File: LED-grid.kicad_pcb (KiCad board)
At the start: 2 copper layers, 75 x 90 mm, 314 parts, among them Q1 NMOS, SW1 SW_Wuerth_450301014042, U1 NE555D, U2 LM741

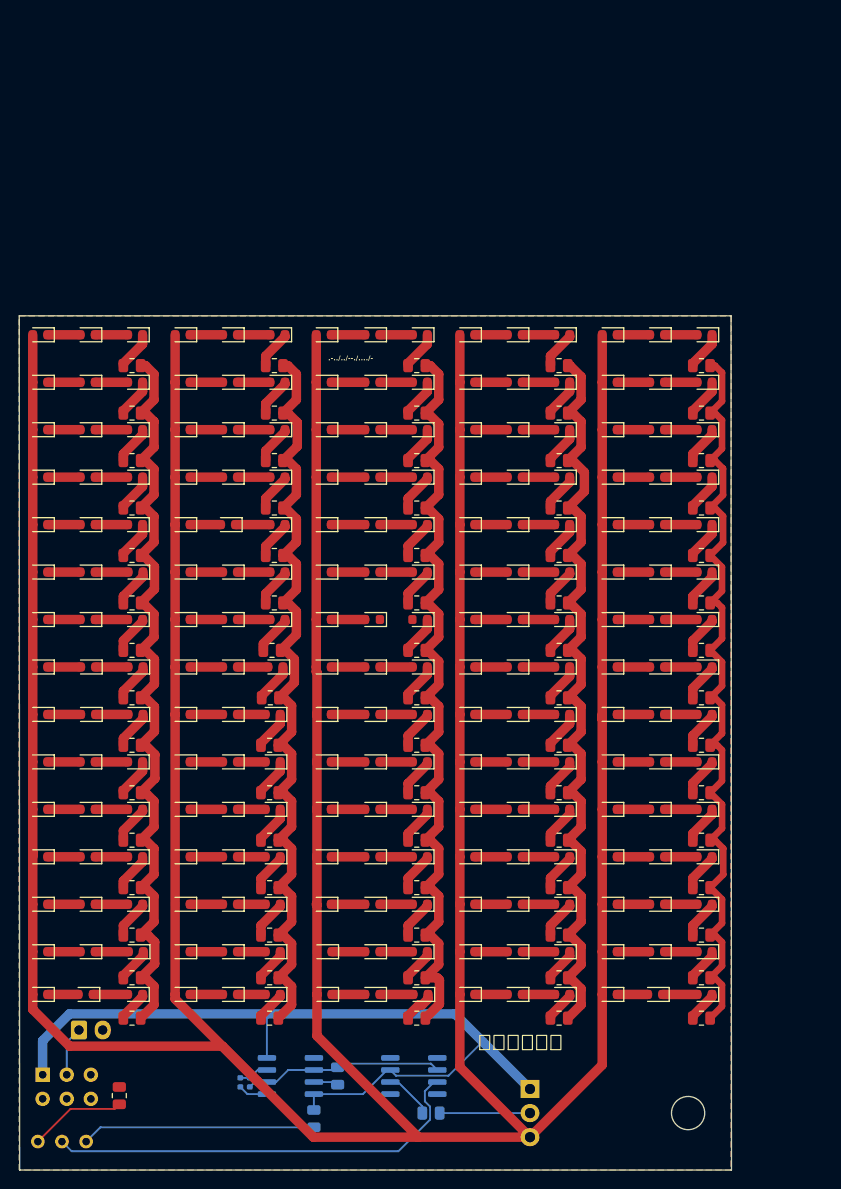
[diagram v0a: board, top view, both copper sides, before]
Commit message: Updated PCB
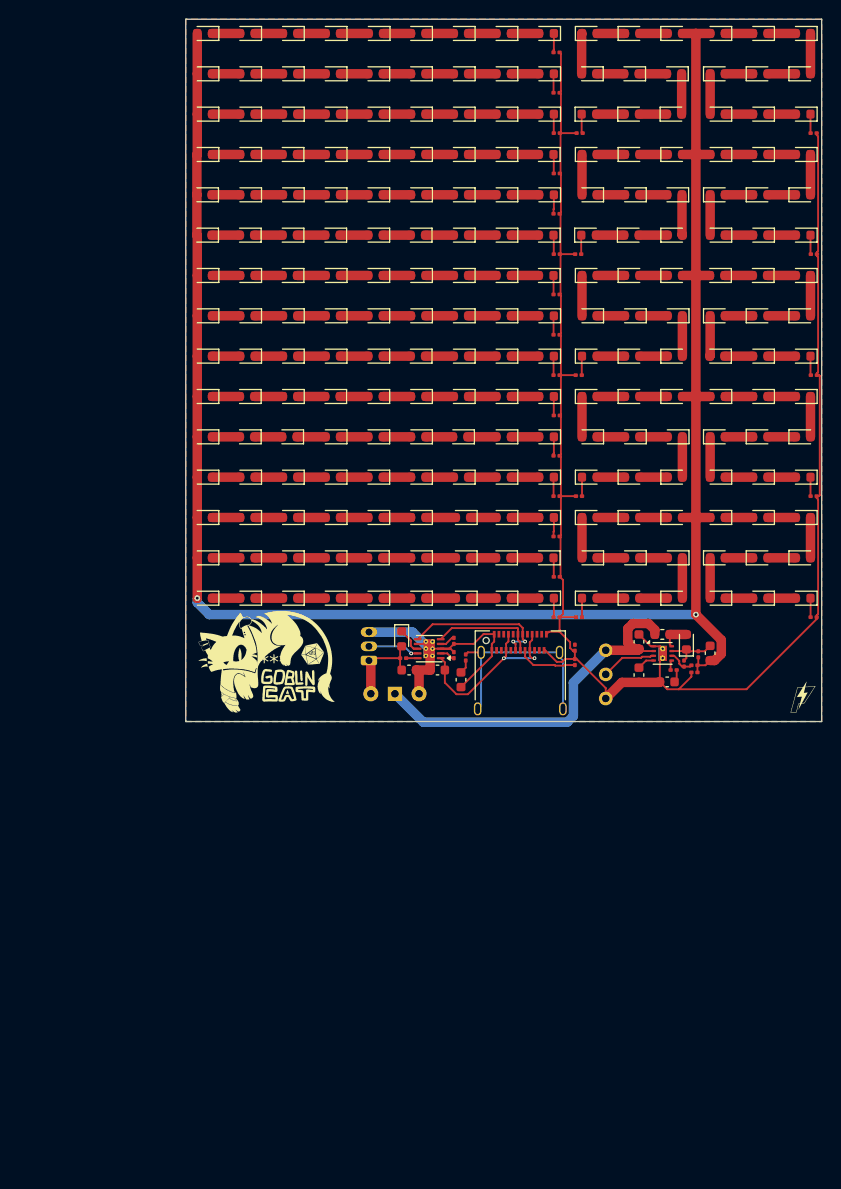
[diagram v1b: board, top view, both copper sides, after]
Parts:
- removed BT1: 6V, Connector_JST:JST_EH_B2B-EH-A_1x02_P2.50mm_Vertical
- removed Q1: NMOS, Package_TO_SOT_THT:TO-220-3_Horizontal_TabUp
- removed R35, R36, R37, R38, R39, R40, R41, R42, R43, R44, R45, R46, R47, R48, R49, R50, R51, R52, R53, R54, R55, R56, R57, R58, R59, R60, R61, R62, R63, R64, R65, R66, R67, R68, R69, R70, R71, R72, R73, R74, R75: 120, Resistor_SMD:R_0805_2012Metric
- removed R76, R77, R78, R79: 1k, Resistor_SMD:R_0805_2012Metric
- removed U2: LM741, Package_SO:SOIC-8_3.9x4.9mm_P1.27mm
- added C3: 1u, Capacitor_SMD:C_0603_1608Metric, F.Cu at (171.0, 92.3)
- added C4: 1u, Capacitor_SMD:C_0603_1608Metric, F.Cu at (195.2, 89.3)
- added C5: 1u, Capacitor_SMD:C_0603_1608Metric, F.Cu at (195.2, 92.8)
- added C6: 10n, Capacitor_SMD:C_0603_1608Metric, F.Cu at (198.2, 93.6)
- added C7: 1n, Capacitor_SMD:C_0201_0603Metric, F.Cu at (200.0, 91.6)
- added C8: 2u, Capacitor_SMD:C_0603_1608Metric, F.Cu at (202.8, 90.5)
- added C9: 47n, Capacitor_SMD:C_0201_0603Metric, F.Cu at (201.1, 92.6)
- added D226: LED, LED_SMD:LED_0603_1608Metric, F.Cu at (208.0, 84.8)
- added D227: LED, LED_SMD:LED_0603_1608Metric, F.Cu at (212.5, 84.8)
- added J1: Conn_01x03_Pin, Connector_JST:JST_ZH_B3B-ZR_1x03_P1.50mm_Vertical, B.Cu at (166.8, 91.3)
- added J2: USB_C_Receptacle, Connector_USB:USB_C_Receptacle_Amphenol_12401610E4-2A, F.Cu at (182.8, 93.6)
- added L1: 30u, Inductor_SMD:L_0603_1608Metric, F.Cu at (197.7, 88.6)
- added U3: BQ24052, Package_SON:WSON-10-1EP_2.5x2.5mm_P0.5mm_EP1.2x2mm_ThermalVias, F.Cu at (173.2, 90.1)
- C1, C2: value 100n -> 1u; footprint Capacitor_SMD:C_0402_1005Metric -> Capacitor_SMD:C_0603_1608Metric; moved to F.Cu
- D2: value LED -> D; footprint LED_SMD:LED_0603_1608Metric -> Diode_SMD:D_0603_1608Metric
- G*** (x2): moved to F.Cu
- R1, R2: value 120 -> 5.1k; footprint Resistor_SMD:R_0805_2012Metric -> Resistor_SMD:R_0201_0603Metric
- R10, R11, R12, R13, R14, R15, R16, R17, R18, R19, R20, R21, R22, R23, R24, R25, R26, R27, R28, R29, R30, R31, R32, R33, R34: value 120 -> 20; footprint Resistor_SMD:R_0805_2012Metric -> Resistor_SMD:R_0201_0603Metric
- R3, R4, R6: value 120 -> 1k; footprint Resistor_SMD:R_0805_2012Metric -> Resistor_SMD:R_0201_0603Metric
- R5: value 120 -> 2k; footprint Resistor_SMD:R_0805_2012Metric -> Resistor_SMD:R_0201_0603Metric
- R7, R8: value 120 -> 100; footprint Resistor_SMD:R_0805_2012Metric -> Resistor_SMD:R_0201_0603Metric
- R9: value 120 -> 1.6; footprint Resistor_SMD:R_0805_2012Metric -> Resistor_SMD:R_0201_0603Metric
- RV1: value 3296X-1-102LF -> 1k
- SW1: footprint Button_Switch_THT:SW_NKK_G1xJP -> Button_Switch_THT:SW_Slide-03_Wuerth-WS-SLTV_10x2.5x6.4_P2.54mm
- U1: value NE555D -> TPS923650D2DRLR; footprint Package_SO:SOIC-8_3.9x4.9mm_P1.27mm -> Package_SON:WSON-8-1EP_2x2mm_P0.5mm_EP0.9x1.6mm_ThermalVias; moved to F.Cu
- moved D183 110.4 mm to (203.5, 25.2)
- moved D184 110.1 mm to (208.0, 25.2)
- moved D196 110.1 mm to (208.0, 42.2), turned to 0 degrees
- moved D185 109.8 mm to (212.5, 25.2)
- moved D186 103.8 mm to (212.5, 29.5), turned to 0 degrees
- moved D197 103.8 mm to (203.5, 42.2), turned to 0 degrees
- moved D187 98.9 mm to (208.0, 29.5), turned to 0 degrees
- moved D211 98.6 mm to (208.0, 63.5)
- moved D212 98.4 mm to (212.5, 63.5)
- moved D198 97.2 mm to (203.5, 46.5)
- moved D199 97.0 mm to (208.0, 46.5)
- moved D200 96.7 mm to (212.5, 46.5)
- moved D138 95.5 mm to (199.0, 25.2), turned to 0 degrees
- moved D188 94.8 mm to (203.5, 29.5), turned to 0 degrees
- moved D213 91.7 mm to (212.5, 67.8), turned to 0 degrees
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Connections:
- C1 pad 1: Net-(U1-CV) -> Net-(C1-Pad1)
- C2 pad 1: Net-(U1-THR) -> VBUS
- D1 pad 2: LED_PWR -> BAT
- D10 pad 2: LED_PWR -> Net-(D10-A)
- D100 pad 2: LED_PWR -> Net-(D100-A)
- D102 pad 2: Net-(D101-K) -> LED_PWR
- D103 pad 2: LED_PWR -> Net-(D102-K)
- D106 pad 2: LED_PWR -> Net-(D105-K)
- D109 pad 2: LED_PWR -> Net-(D108-K)
- D111 pad 2: Net-(D110-K) -> LED_PWR
- D112 pad 2: LED_PWR -> Net-(D111-K)
- D115 pad 2: LED_PWR -> Net-(D114-K)
- D118 pad 2: LED_PWR -> Net-(D117-K)
- D12 pad 2: Net-(D11-K) -> LED_PWR
- D120 pad 2: Net-(D119-K) -> LED_PWR
- D121 pad 2: LED_PWR -> Net-(D120-K)
- D124 pad 2: LED_PWR -> Net-(D123-K)
- D127 pad 2: LED_PWR -> Net-(D126-K)
- D129 pad 2: Net-(D128-K) -> LED_PWR
- D13 pad 2: LED_PWR -> Net-(D12-K)
- D130 pad 2: LED_PWR -> Net-(D129-K)
- D133 pad 2: LED_PWR -> Net-(D132-K)
- D136 pad 2: LED_PWR -> Net-(D135-K)
- D138 pad 2: Net-(D137-K) -> LED_PWR
- D139 pad 2: LED_PWR -> Net-(D138-K)
- D142 pad 2: LED_PWR -> Net-(D141-K)
- D145 pad 2: LED_PWR -> Net-(D144-K)
- D147 pad 2: Net-(D146-K) -> LED_PWR
- D148 pad 2: LED_PWR -> Net-(D147-K)
- D151 pad 2: LED_PWR -> Net-(D150-K)
- D154 pad 2: LED_PWR -> Net-(D153-K)
- D156 pad 2: Net-(D155-K) -> LED_PWR
- D157 pad 2: LED_PWR -> Net-(D156-K)
- D16 pad 2: LED_PWR -> Net-(D15-K)
- D160 pad 2: LED_PWR -> Net-(D159-K)
- D163 pad 2: LED_PWR -> Net-(D162-K)
- D165 pad 2: Net-(D164-K) -> LED_PWR
- D166 pad 2: LED_PWR -> Net-(D165-K)
- D169 pad 2: LED_PWR -> Net-(D168-K)
- D172 pad 2: LED_PWR -> Net-(D171-K)
- D174 pad 2: Net-(D173-K) -> LED_PWR
- D175 pad 2: LED_PWR -> Net-(D174-K)
- D178 pad 2: LED_PWR -> Net-(D177-K)
- D181 pad 2: LED_PWR -> Net-(D180-K)
- D183 pad 2: Net-(D182-K) -> LED_PWR
- D184 pad 2: LED_PWR -> Net-(D183-K)
- D187 pad 2: LED_PWR -> Net-(D186-K)
- D19 pad 2: LED_PWR -> Net-(D18-K)
- D190 pad 2: LED_PWR -> Net-(D189-K)
- D192 pad 2: Net-(D191-K) -> LED_PWR
- D193 pad 2: LED_PWR -> Net-(D192-K)
- D196 pad 2: LED_PWR -> Net-(D195-K)
- D199 pad 2: LED_PWR -> Net-(D198-K)
- D2 pad 2: Net-(D1-K) -> Net-(D2-A)
- D201 pad 2: Net-(D200-K) -> LED_PWR
- D202 pad 2: LED_PWR -> Net-(D201-K)
- D205 pad 2: LED_PWR -> Net-(D204-K)
- D208 pad 2: LED_PWR -> Net-(D207-K)
- D21 pad 2: Net-(D20-K) -> LED_PWR
- D210 pad 2: Net-(D209-K) -> LED_PWR
- D211 pad 2: LED_PWR -> Net-(D210-K)
- D214 pad 2: LED_PWR -> Net-(D213-K)
- D217 pad 2: LED_PWR -> Net-(D216-K)
- D219 pad 2: Net-(D218-K) -> LED_PWR
- D22 pad 2: LED_PWR -> Net-(D21-K)
- D220 pad 2: LED_PWR -> Net-(D219-K)
- D223 pad 2: LED_PWR -> Net-(D222-K)
- D25 pad 2: LED_PWR -> Net-(D24-K)
- D28 pad 2: LED_PWR -> Net-(D27-K)
- D3 pad 2: Net-(D2-K) -> LED_PWR
- D30 pad 2: Net-(D29-K) -> LED_PWR
- D31 pad 2: LED_PWR -> Net-(D30-K)
- D34 pad 2: LED_PWR -> Net-(D33-K)
- D37 pad 2: LED_PWR -> Net-(D36-K)
- D39 pad 2: Net-(D38-K) -> LED_PWR
- D4 pad 2: LED_PWR -> Net-(D3-K)
- D40 pad 2: LED_PWR -> Net-(D39-K)
- D43 pad 2: LED_PWR -> Net-(D42-K)
- D46 pad 2: LED_PWR -> Net-(D45-K)
- D48 pad 2: Net-(D47-K) -> LED_PWR
- D49 pad 2: LED_PWR -> Net-(D48-K)
- D52 pad 2: LED_PWR -> Net-(D51-K)
- D55 pad 2: LED_PWR -> Net-(D54-K)
- D57 pad 2: Net-(D56-K) -> LED_PWR
- D58 pad 2: LED_PWR -> Net-(D57-K)
- D61 pad 2: LED_PWR -> Net-(D60-K)
- D64 pad 2: LED_PWR -> Net-(D63-K)
- D66 pad 2: Net-(D65-K) -> LED_PWR
- D67 pad 2: LED_PWR -> Net-(D66-K)
- D7 pad 2: LED_PWR -> Net-(D6-K)
- D70 pad 2: LED_PWR -> Net-(D69-K)
- D73 pad 2: LED_PWR -> Net-(D72-K)
- D75 pad 2: Net-(D74-K) -> LED_PWR
- D76 pad 2: LED_PWR -> Net-(D75-K)
- D79 pad 2: LED_PWR -> Net-(D78-K)
- D82 pad 2: LED_PWR -> Net-(D81-K)
- D84 pad 2: Net-(D83-K) -> LED_PWR
- D85 pad 2: LED_PWR -> Net-(D84-K)
- D88 pad 2: LED_PWR -> Net-(D87-K)
- D9 pad 1: Net-(D9-K) -> Net-(D10-A)
- D91 pad 2: LED_PWR -> Net-(D90-K)
- D93 pad 2: Net-(D92-K) -> LED_PWR
- D94 pad 2: LED_PWR -> Net-(D93-K)
- D97 pad 2: LED_PWR -> Net-(D96-K)
- D99 pad 1: Net-(D99-K) -> Net-(D100-A)
- R1 pad 1: Net-(D3-K) -> Net-(J2-CC1)
- R10 pad 1: Net-(D30-K) -> Net-(D11-K)
- R11 pad 1: Net-(D33-K) -> Net-(D20-K)
- R12 pad 1: Net-(D36-K) -> Net-(D29-K)
- R13 pad 1: Net-(D39-K) -> Net-(D38-K)
- R14 pad 1: Net-(D42-K) -> Net-(D47-K)
- R15 pad 1: Net-(D45-K) -> Net-(D56-K)
- R16 pad 1: Net-(D48-K) -> Net-(D65-K)
- R17 pad 1: Net-(D51-K) -> Net-(D74-K)
- R18 pad 1: Net-(D54-K) -> Net-(D83-K)
- R19 pad 1: Net-(D57-K) -> Net-(D92-K)
- R2 pad 1: Net-(D6-K) -> Net-(J2-CC2)
- R20 pad 1: Net-(D60-K) -> Net-(D101-K)
- R21 pad 1: Net-(D63-K) -> Net-(D110-K)
- R22 pad 1: Net-(D66-K) -> Net-(D119-K)
- R23 pad 1: Net-(D69-K) -> Net-(D128-K)
- R24 pad 1: Net-(D72-K) -> Net-(D137-K)
- R25 pad 1: Net-(D75-K) -> Net-(D146-K)
- R26 pad 1: Net-(D78-K) -> Net-(D155-K)
- R27 pad 1: Net-(D81-K) -> Net-(D164-K)
- R28 pad 1: Net-(D84-K) -> Net-(D173-K)
- R29 pad 1: Net-(D87-K) -> Net-(D182-K)
- R3 pad 1: Net-(D9-K) -> Net-(J2-SHIELD)
- R3 pad 2: GND -> Net-(C1-Pad1)
- R30 pad 1: Net-(D90-K) -> Net-(D191-K)
- R31 pad 1: Net-(D93-K) -> Net-(D200-K)
- R32 pad 1: Net-(D96-K) -> Net-(D209-K)
- R33 pad 1: Net-(D99-K) -> Net-(D218-K)
- R34 pad 1: Net-(D102-K) -> Net-(D227-K)
- R4 pad 1: Net-(D12-K) -> GND
- R4 pad 2: GND -> Net-(U3-ISET)
- R5 pad 1: Net-(D15-K) -> GND
- R5 pad 2: GND -> Net-(U3-PRE-TERM)
- R6 pad 1: Net-(D18-K) -> Net-(U3-OUT)
- R6 pad 2: GND -> BAT
- R7 pad 1: Net-(D21-K) -> Net-(U1-COMP)
- R7 pad 2: GND -> Net-(C6-Pad1)
- R8 pad 1: Net-(D24-K) -> Net-(U1-CSN)
- R8 pad 2: GND -> LED_PWR
- R9 pad 1: Net-(D27-K) -> Net-(D2-K)
- R9 pad 2: GND -> LED_PWR
- RV1 pad 1: Net-(R77-Pad1) -> VCC
- RV1 pad 2: Net-(U2-+) -> Net-(U1-DIM)
- RV1 pad 3: Net-(R78-Pad2) -> GND
- SW1 pad 2: Net-(BT1-+) -> GND
- SW1 pad 3: GND -> BAT
- U1 pad 2: Net-(U1-THR) -> VCC
- U1 pad 3: Net-(U1-Q) -> Net-(U1-DIM)
- U1 pad 4: VCC -> Net-(U1-VCC)
- U1 pad 5: Net-(U1-CV) -> Net-(U1-COMP)
- U1 pad 6: Net-(U1-THR) -> Net-(U1-CSN)
- U1 pad 7: GND -> Net-(D2-K)
- U1 pad 8: VCC -> Net-(D2-A)
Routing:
- net LED_PWR: track 476.8 -> 198.7 mm, vias 0 -> 2
- net GND: track 447.0 -> 202.3 mm
- net VCC: track 87.4 -> 40.6 mm
- net Net-(U2-+): track 45.5 -> 0.00 mm
- net Net-(R77-Pad1): track 24.6 -> 0.00 mm
- net Net-(J2-SHIELD): track 0.00 -> 22.2 mm
- net Net-(U1-THR): track 21.0 -> 0.00 mm
- net VBUS: track 0.00 -> 20.0 mm, vias 0 -> 2
- net USB_D-: track 0.00 -> 15.7 mm, vias 0 -> 2
- net USB_D+: track 0.00 -> 11.0 mm
- net BAT: track 0.00 -> 10.3 mm
- net Net-(R78-Pad2): track 10.2 -> 0.00 mm
- net Net-(Q1-G): track 9.52 -> 0.00 mm
- net Net-(J2-CC2): track 0.00 -> 6.34 mm
- net Net-(U1-DIM): track 0.00 -> 5.86 mm
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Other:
- board size 75 x 90 mm -> 67 x 74 mm
- board text removed: ".-../../--./..../-"
- board text removed: "A PiShock product"
- board text removed: "Designed by:"
- board text removed: "FLASHBANG v1.0.1"
- board text removed: "GitHub: dorythecat Discord: dorythecat"
- board text removed: "Lights, camera, action!"
- board text removed: "R20"
- board text removed: "手が痛かった"
